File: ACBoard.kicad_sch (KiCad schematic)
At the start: 25 parts, among them J1 Conn_02x20_Odd_Even, J2 Conn_02x20_Odd_Even, J3 Conn_01x02_Male, J4 Conn_01x02_Female, J5 Conn_01x02_Female, T1 CSE185L, U1 TLP561, U2 TLP561, U3 ADS7822U

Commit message: Update ACBoard.kicad_sch
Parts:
- R5: footprint Resistor_SMD:R_0603_1608Metric_Pad0.98x0.95mm_HandSolder -> Resistor_SMD:R_2010_5025Metric_Pad1.40x2.65mm_HandSolder
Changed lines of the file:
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@@
       (effects (font (size 1.27 1.27)) (justify left))
     )
-    (property "Footprint" "Resistor_SMD:R_0603_1608Metric_Pad0.98x0.95mm_HandSolder" (id 2) (at 202.692 63.5 90)
+    (property "Footprint" "Resistor_SMD:R_2010_5025Metric_Pad1.40x2.65mm_HandSolder" (id 2) (at 202.692 63.5 90)
       (effects (font (size 1.27 1.27)) hide)
     )
@@
     )
     (path "/0d402606-3120-4980-8456-8f91cb64a988"
-      (reference "R5") (unit 1) (value "67") (footprint "Resistor_SMD:R_0603_1608Metric_Pad0.98x0.95mm_HandSolder")
+      (reference "R5") (unit 1) (value "67") (footprint "Resistor_SMD:R_2010_5025Metric_Pad1.40x2.65mm_HandSolder")
     )
     (path "/fe4fefbf-4e6d-41f6-b3b2-a9a978e16f7d"

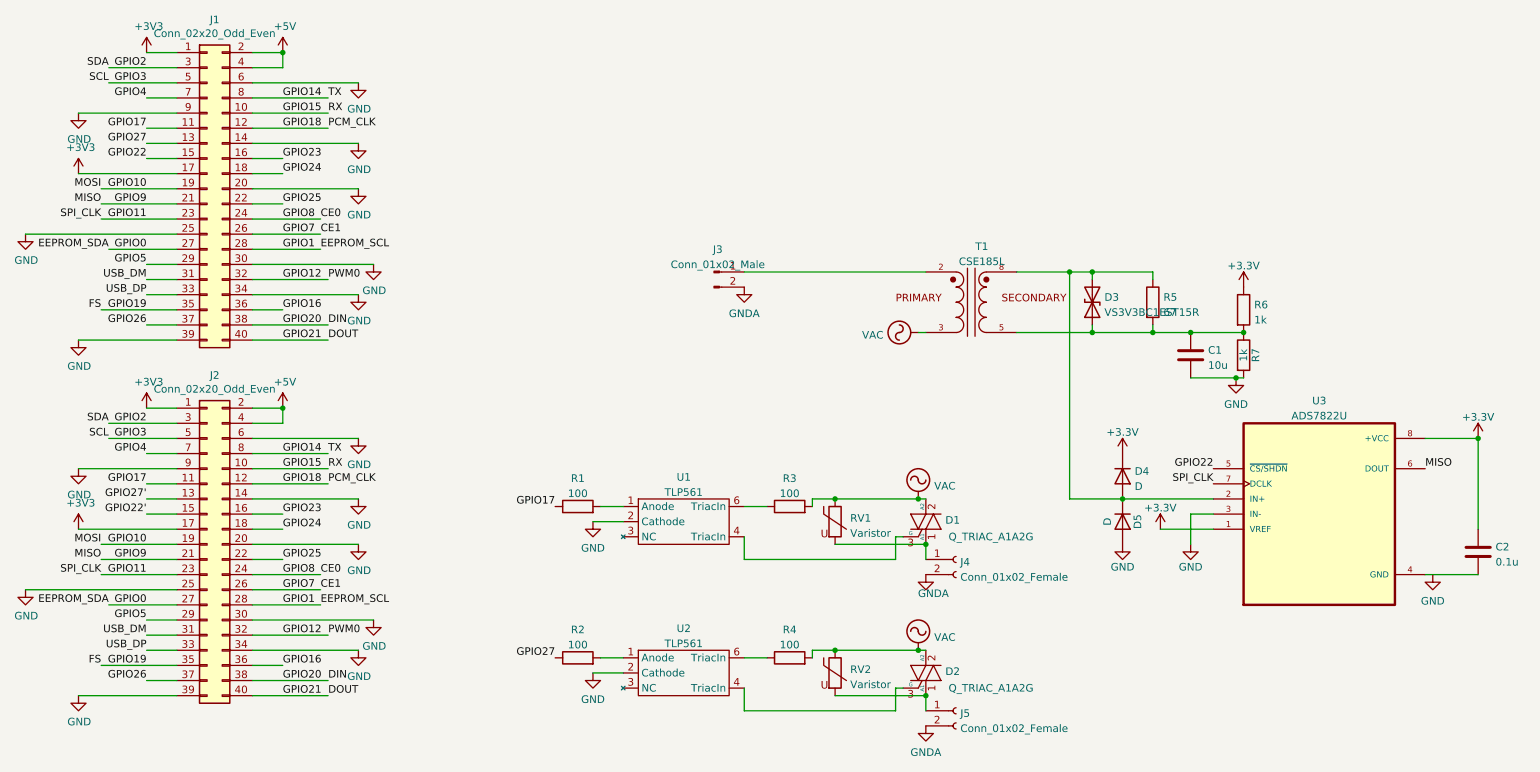
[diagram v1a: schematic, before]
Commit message: data19
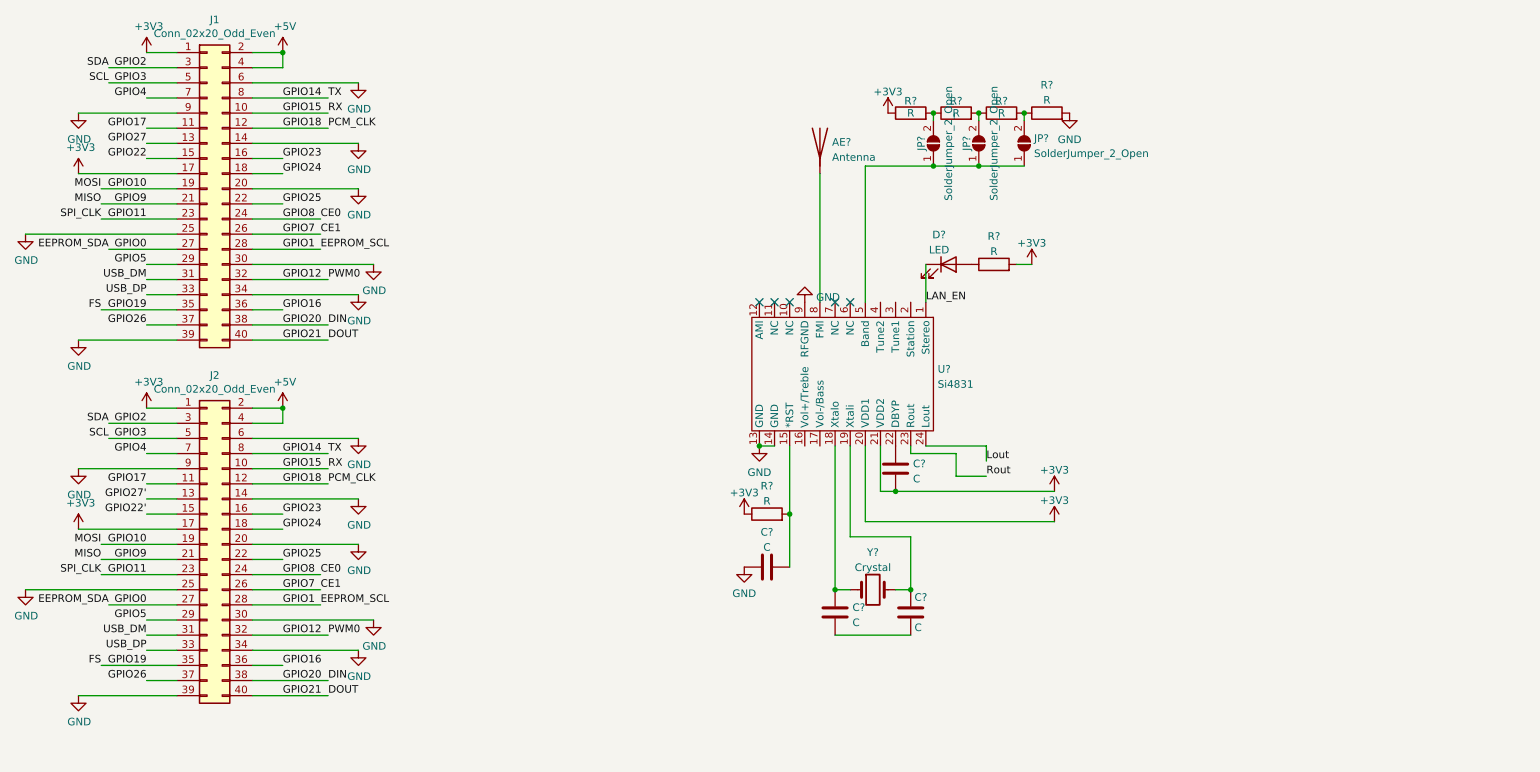
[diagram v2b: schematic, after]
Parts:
- removed C1: 10u, Capacitor_SMD:C_0805_2012Metric_Pad1.18x1.45mm_HandSolder, symbol Device:C
- removed C2: 0.1u, Capacitor_SMD:C_1206_3216Metric_Pad1.33x1.80mm_HandSolder, symbol Device:C
- removed D1, D2: Q_TRIAC_A1A2G, Package_TO_SOT_THT:TO-220-3_Horizontal_TabDown, symbol Device:Q_TRIAC_A1A2G
- removed D3: VS3V3BC1EST15R, Diode_SMD:D_0201_0603Metric_Pad0.64x0.40mm_HandSolder, symbol Device:D_TVS
- removed D4, D5: D, Diode_THT:D_5W_P12.70mm_Horizontal, symbol Device:D
- removed J3: Conn_01x02_Male, locallib:ACinlet, symbol Connector:Conn_01x02_Male
- removed J4, J5: Conn_01x02_Female, locallib:AcOutlet, symbol Connector:Conn_01x02_Female
- removed R1, R2, R3, R4: 100, Resistor_SMD:R_0603_1608Metric_Pad0.98x0.95mm_HandSolder, symbol Device:R
- removed R5: 67, Resistor_SMD:R_2010_5025Metric_Pad1.40x2.65mm_HandSolder, symbol Device:R
- removed R6, R7: 1k, Resistor_SMD:R_0603_1608Metric_Pad0.98x0.95mm_HandSolder, symbol Device:R
- removed RV1, RV2: Varistor, Varistor:RV_Disc_D9mm_W3.8mm_P5mm, symbol Device:Varistor
- removed T1: CSE185L, locallib:XFMR_CSE185L, symbol locallib:CSE185L
- removed U1, U2: TLP561, Package_DIP:DIP-5-6_W7.62mm, symbol locallib:TLP561
- removed U3: ADS7822U, locallib:SOIC127P599X175-8N, symbol locallib:ADS7822U
- added AE?: Antenna, symbol Device:Antenna
- added C? (x4): C, symbol Device:C
- added D?: LED, symbol Device:LED
- added JP? (x3): SolderJumper_2_Open, symbol Jumper:SolderJumper_2_Open
- added R? (x6): R, symbol Device:R
- added U?: Si4831, symbol locallib:Si4831
- added Y?: Crystal, symbol Device:Crystal
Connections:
- net +3V3: now also C?.2, R?.1, R?.1, R?.2, U?.20 (VDD1), U?.21 (VDD2)
- net GND: now also C?.1, R?.2, U?.13 (GND), U?.14 (GND), U?.9 (RFGND)
- new net: JP?.2 (B), R?.1, R?.2 (x3)
- new net: C?.2, R?.2, U?.15 (*RST)
- new net: AE?.1 (A), U?.8 (FMI)
- new net: C?.1, U?.22 (DBYP)
- new net: C?.1, U?.18 (Xtalo), Y?.1
- new net: C?.2, C?.2
- new net: C?.1, U?.19 (Xtali), Y?.2
- new net: JP?.1 (A), JP?.1 (A), JP?.1 (A), U?.5 (Band)
- new net: D?.2 (A), R?.1
- new net LAN_EN: D?.1 (K), U?.1 (Stereo)
- new net Lout: U?.24 (Lout)
- new net Rout: U?.23 (Rout)
- no-connect marks 0 -> 5
